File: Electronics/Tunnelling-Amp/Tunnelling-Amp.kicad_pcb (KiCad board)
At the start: 2 copper layers, 49.8 x 19.8 mm, 19 parts, among them J1 RF_Shield_Two_Pieces, U1 ADA4637-1

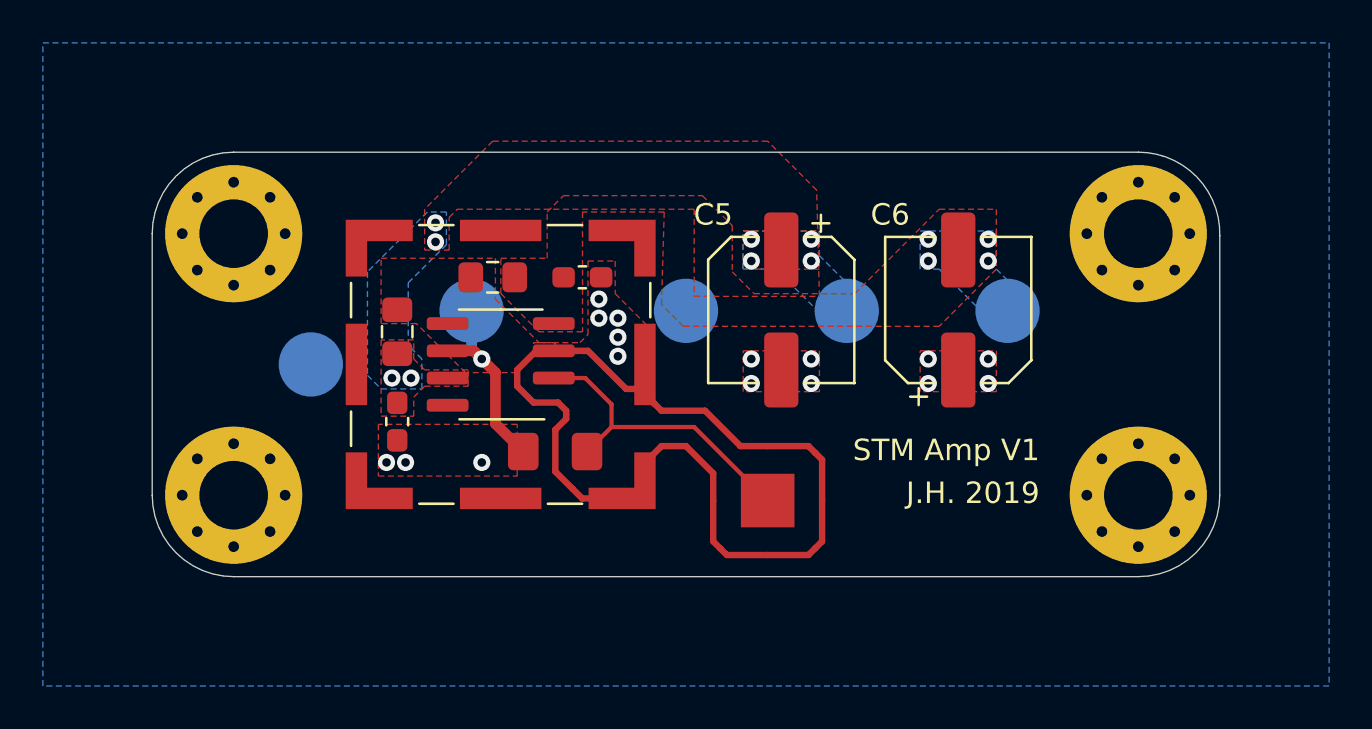
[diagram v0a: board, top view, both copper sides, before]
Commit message: Power Supply Design Requirements
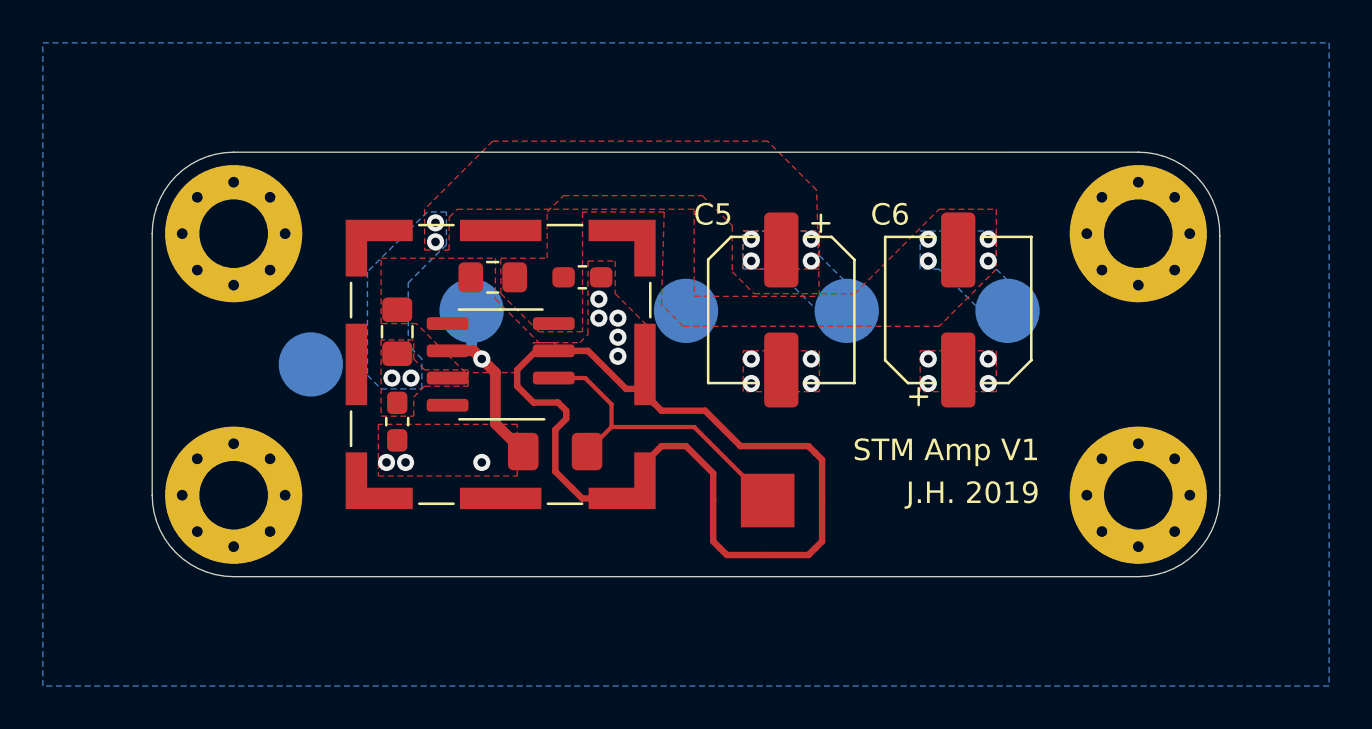
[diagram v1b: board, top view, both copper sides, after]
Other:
- net class Default removed
